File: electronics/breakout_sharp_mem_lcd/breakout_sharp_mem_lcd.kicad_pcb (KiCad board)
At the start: 2 copper layers, 26 x 18 mm, 12 parts, among them J1 Conn_01x06, J2 Conn_01x10

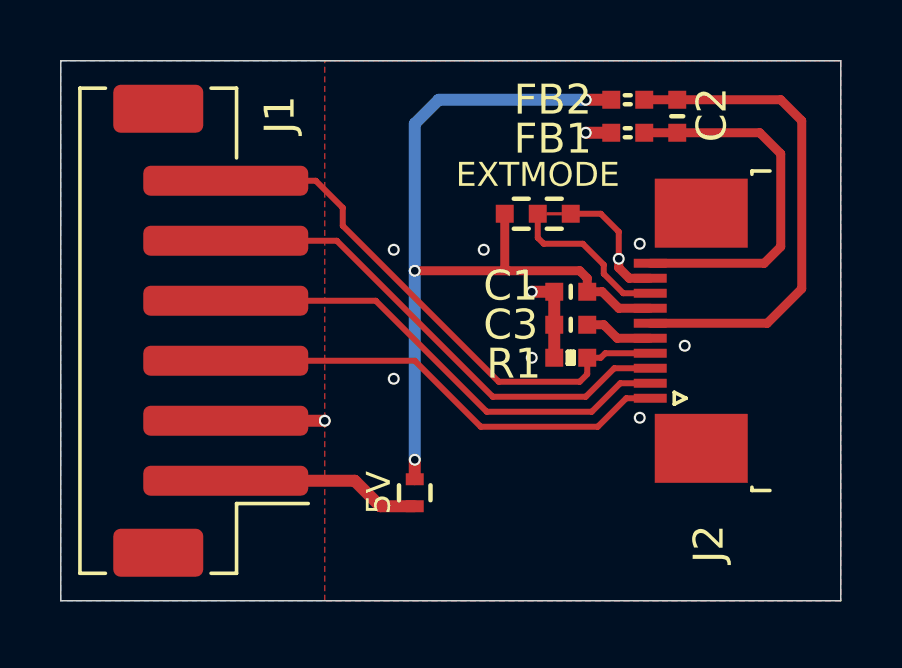
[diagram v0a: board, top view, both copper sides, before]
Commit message: placed, routed, silk placed, optimized
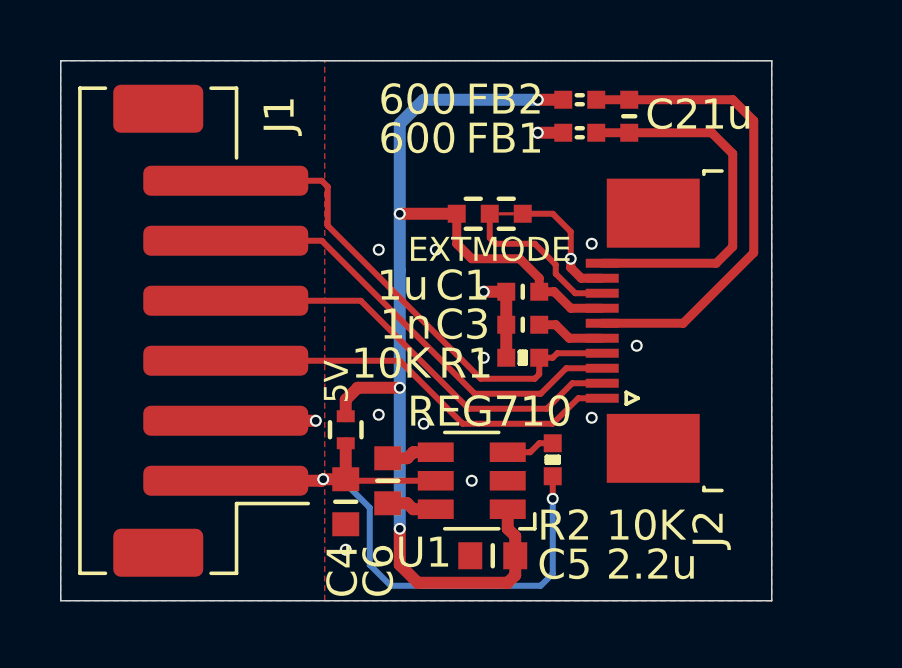
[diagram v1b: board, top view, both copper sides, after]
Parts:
- added C4: 2.2u, SquantorRcl:C_0603, F.Cu at (146.5, 76.7)
- added C5: 2.2u, SquantorRcl:C_0603, F.Cu at (151.4, 78.5)
- added C6: 0.22u, SquantorRcl:C_0603, F.Cu at (147.9, 76.0)
- added R2: 10K, SquantorRcl:R_0402_hand, F.Cu at (153.4, 75.3)
- added U1: REG710, SquantorIC:SOT23-6-HAND, F.Cu at (150.7, 76.0)
- N1: value 20210913 -> 20210927
- moved JP2 3.11 mm to (146.5, 74.3)
- moved C2 1.60 mm to (155.9, 63.9)
- moved C1 1.60 mm to (152.4, 69.7)
- moved C3 1.60 mm to (152.4, 70.8)
- moved FB1 1.60 mm to (154.3, 64.4)
- moved FB2 1.60 mm to (154.3, 63.3)
- moved J2 1.60 mm to (156.4, 71.0)
- moved JP1 1.60 mm to (151.3, 67.1)
- moved R1 1.60 mm to (152.4, 71.9)
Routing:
- net /VDD_IN: track 6.65 -> 21.9 mm, vias 0 -> 2
- net /VDD: track 29.3 -> 38.4 mm, vias 3 -> 4
- net /SCS: track 16.7 -> 15.0 mm
- net /SCLK: track 15.5 -> 13.8 mm
- net /SI: track 16.1 -> 14.4 mm
- net Net-(C6-Pad2): track 0.00 -> 1.68 mm
- net Net-(C6-Pad1): track 0.00 -> 1.68 mm
- net Net-(R2-Pad1): track 0.00 -> 1.62 mm
- net /EXTCOMIN: track 18.0 -> 16.7 mm
- net /VDDA: track 16.7 -> 16.0 mm
- net /VSS: track 11.3 -> 11.0 mm, vias 11 -> 14
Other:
- board size 26 x 18 mm -> 23.7 x 18 mm
